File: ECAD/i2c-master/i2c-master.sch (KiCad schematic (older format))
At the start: 19 parts, among them J1 Conn_01x12_Female, J10 Conn_01x05, J11 Barrel_Jack, J12 Conn_02x10_Odd_Even, J2 Conn_01x05, J3 Conn_01x05, J4 Conn_01x05, J5 Conn_01x05, J6 Conn_01x12_Female, J7 Conn_01x05, J8 Conn_01x05, J9 Conn_01x05, U1 L7805

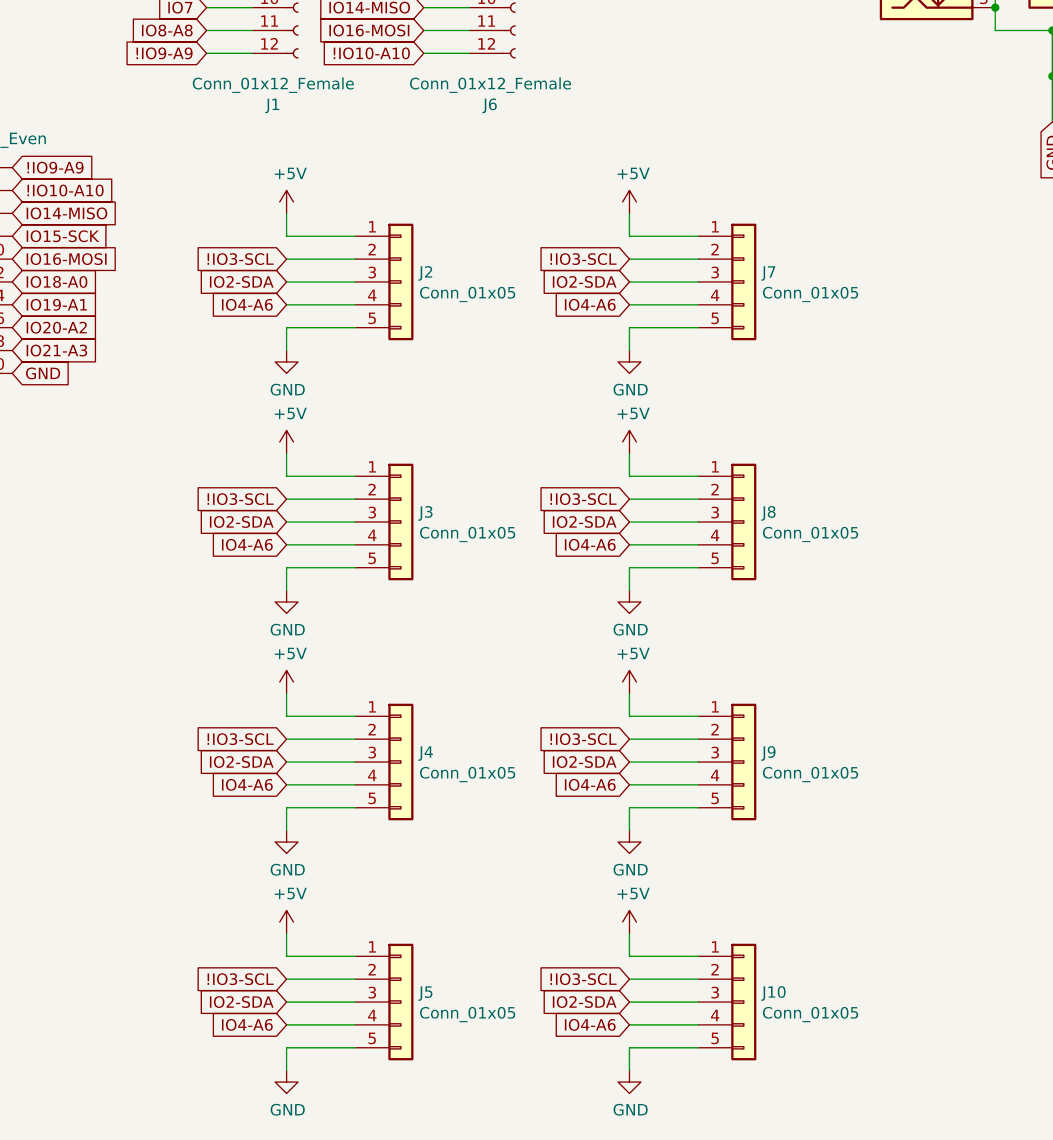
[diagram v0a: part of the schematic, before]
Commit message: Whoops, forgot the master board
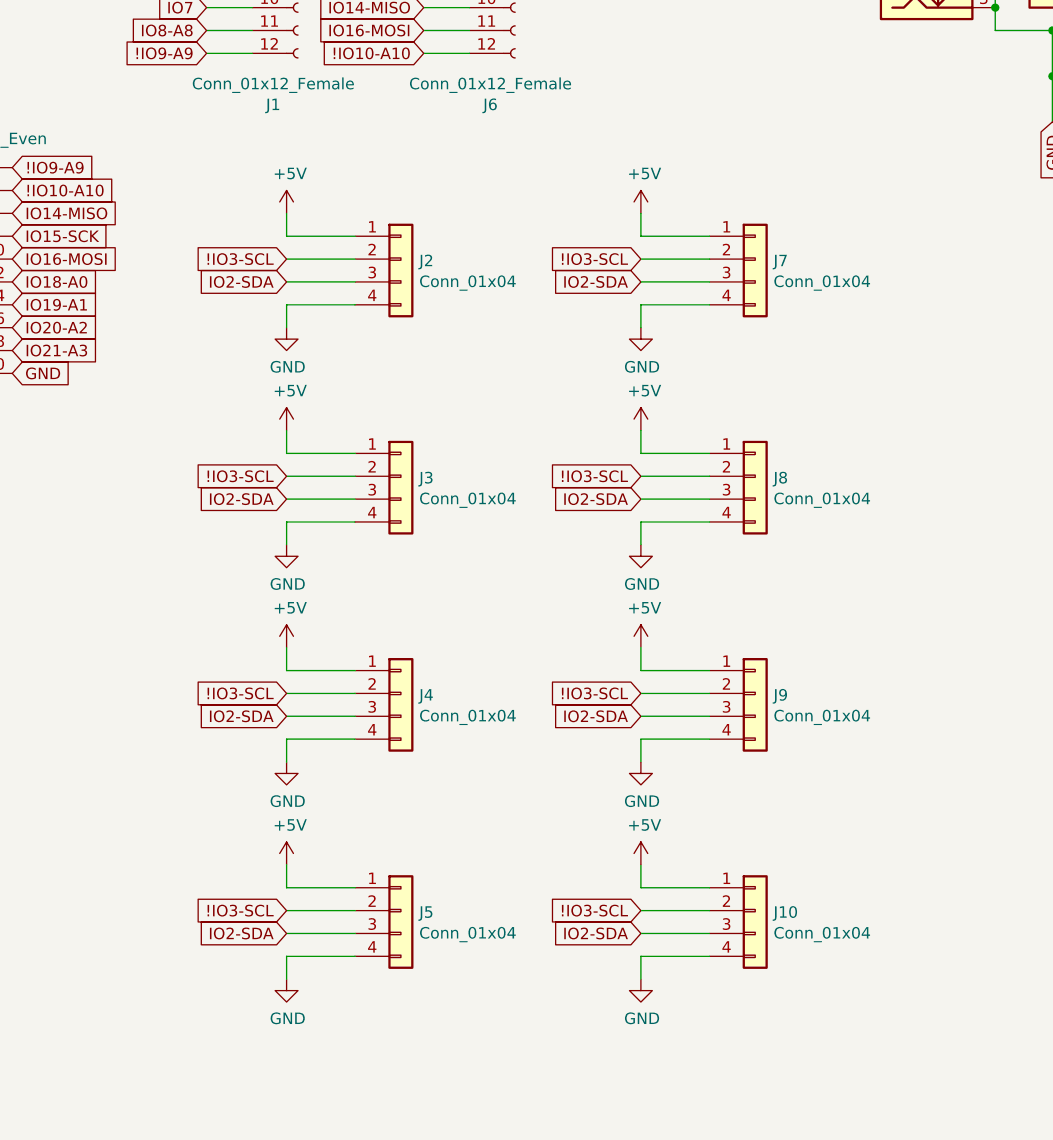
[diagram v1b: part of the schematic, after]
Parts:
- removed J10, J2, J3, J4, J5, J7, J8, J9: Conn_01x05, Connector_JST:JST_GH_BM05B-GHS-TBT_1x05-1MP_P1.25mm_Vertical, symbol Connector_Generic:Conn_01x05
- added J10, J2, J3, J4, J5, J7, J8, J9: Conn_01x04, Connector_JST:JST_GH_BM04B-GHS-TBT_1x04-1MP_P1.25mm_Vertical, symbol Connector_Generic:Conn_01x04
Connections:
- net !IO3-SCL: now also J10.2 (Pin_2), J2.2 (Pin_2), J3.2 (Pin_2), J4.2 (Pin_2), J5.2 (Pin_2), J7.2 (Pin_2), J8.2 (Pin_2), J9.2 (Pin_2)
- net +5V: now also J10.1 (Pin_1), J2.1 (Pin_1), J3.1 (Pin_1), J4.1 (Pin_1), J5.1 (Pin_1), J7.1 (Pin_1), J8.1 (Pin_1), J9.1 (Pin_1)
- net GND: now also J10.4 (Pin_4), J2.4 (Pin_4), J3.4 (Pin_4), J4.4 (Pin_4), J5.4 (Pin_4), J7.4 (Pin_4), J8.4 (Pin_4), J9.4 (Pin_4)
- net IO2-SDA: now also J10.3 (Pin_3), J2.3 (Pin_3), J3.3 (Pin_3), J4.3 (Pin_3), J5.3 (Pin_3), J7.3 (Pin_3), J8.3 (Pin_3), J9.3 (Pin_3)
